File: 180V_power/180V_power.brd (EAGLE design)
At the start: 50 x 75 mm, 22 parts, among them IC1 NE555P, Q1 IRF740S, Q2 BC546

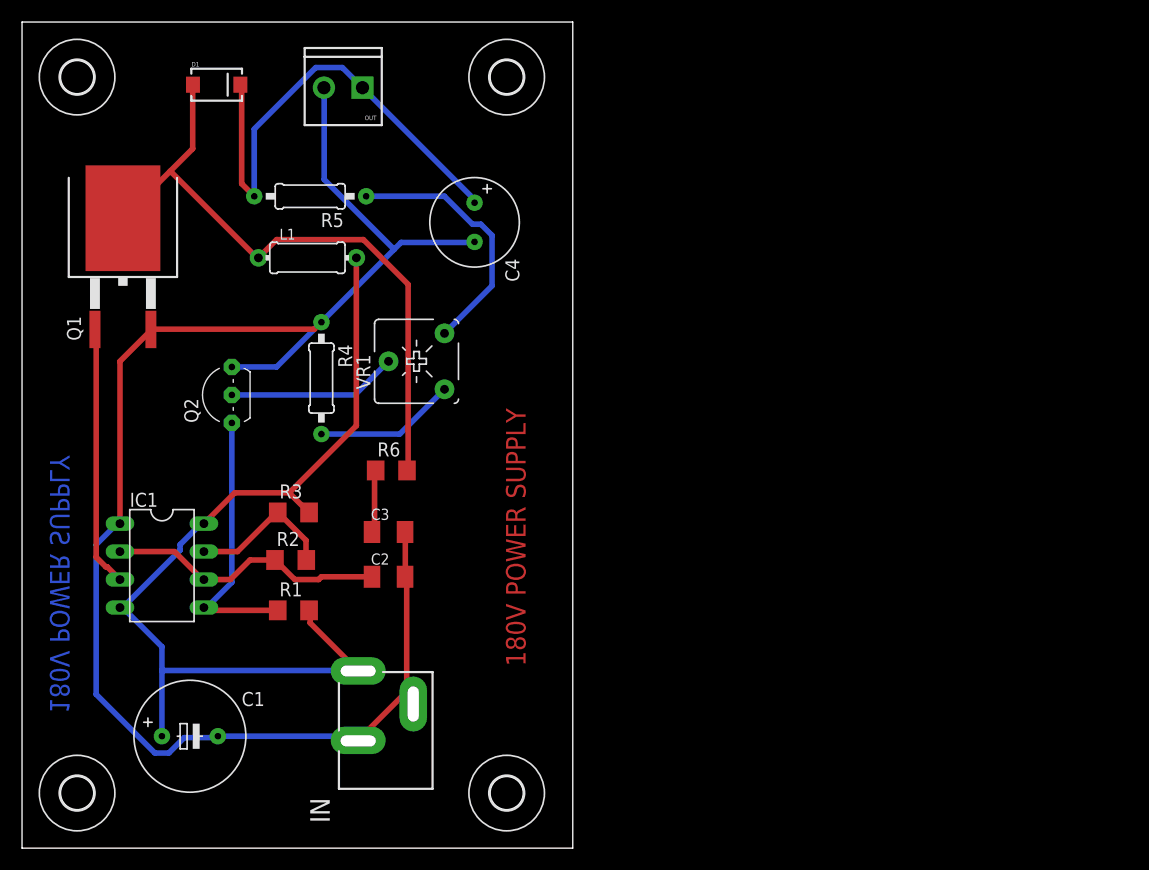
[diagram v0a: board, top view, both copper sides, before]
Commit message: new simple 180 board
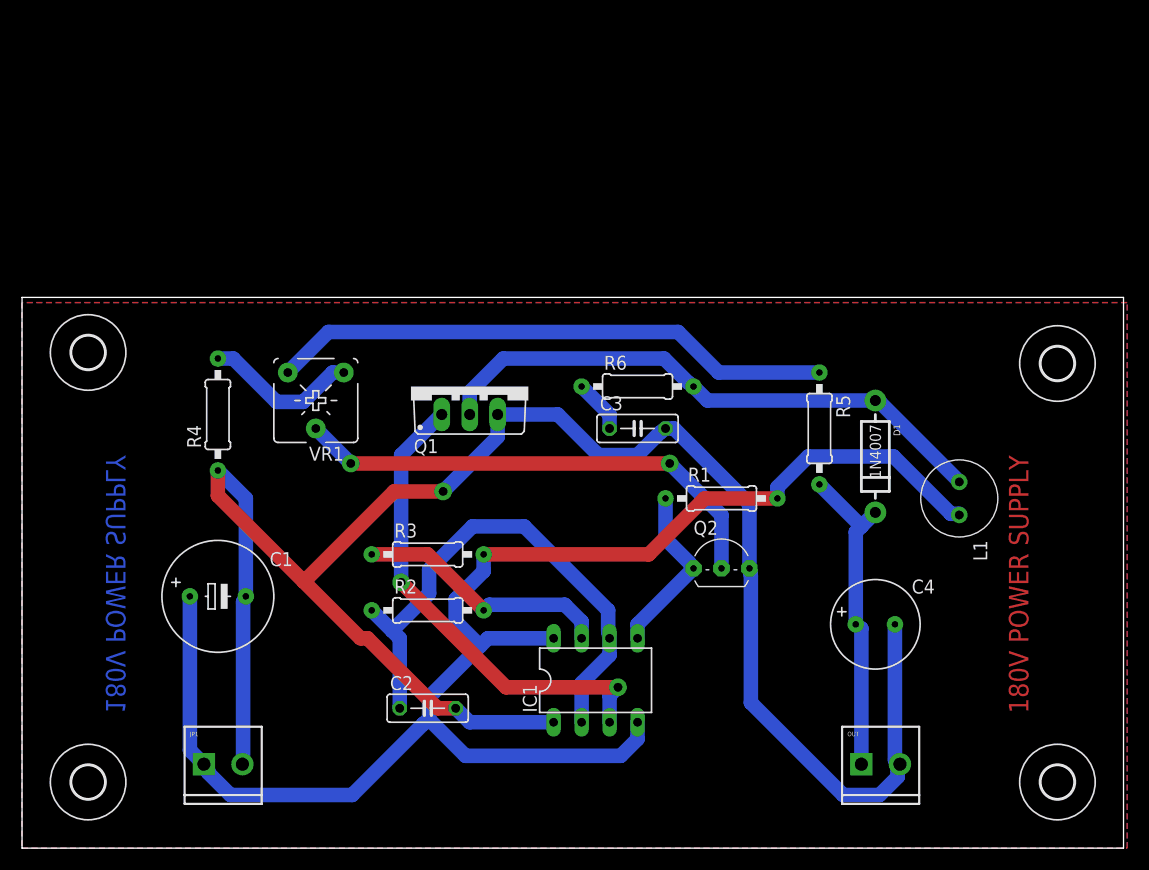
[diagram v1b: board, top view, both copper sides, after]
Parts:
- removed IN: POWER_JACKSLT, iStivi - Header-Connector:POWER_JACK_SLOT
- added JP1: (no value), iStivi - Header-Connector:SCREWTERMINAL-3.5MM-2
- C2, C3: device iStivi - RCLD:C1206K -> iStivi - RCLD:C050-025X075
- D1: device iStivi - RCLD:SMA-DIODE -> iStivi - RCLD:DIODE-1N4001
- L1: value 100uH -> (none); device iStivi - RCLD:TFI0307 -> iStivi - RCLD:RBL0712
- Q1: value IRF740S -> IRF740; device iStivi - Transistor-FET:TO263 -> iStivi - Transistor-FET:TO220BV
- R1, R2, R3, R6: device iStivi - RCLD:R1206 -> iStivi - RCLD:0207/10
- moved OUT 76.3 mm to (76.2, 7.62), turned to 0 degrees
- moved D1 68.7 mm to (77.5, 35.6), turned to 270 degrees
- moved L1 63.1 mm to (85.1, 31.8), turned to 270 degrees
- moved U$3 56.4 mm to (94.0, 44.0)
- moved C4 51.5 mm to (77.5, 20.3), turned to 0 degrees
- moved R5 50.8 mm to (72.4, 38.1), turned to 270 degrees
- moved U$2 50.0 mm to (94.0, 6.00)
- moved Q2 48.0 mm to (63.5, 26.7), turned to 0 degrees
- moved IC1 40.7 mm to (52.1, 15.2), turned to 0 degrees
- moved R1 40.2 mm to (63.5, 31.8)
- moved Q1 33.6 mm to (40.6, 41.9)
- moved U$4 25.0 mm to (6.00, 45.0)
- moved C3 24.5 mm to (55.9, 38.1)
- moved R6 23.6 mm to (55.9, 41.9)
- moved R2 13.3 mm to (36.8, 21.6)
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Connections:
- net GND: now also JP1.2, Q1.S; no longer IN.GND@1, IN.GND@2, Q1.2
- net N$1: now also Q1.G; no longer Q1.1
- net N$26: now also JP1.1, L1.P$2; no longer IN.PWR, L1.2
- net N$6: now also L1.P$1, Q1.D; no longer L1.1, Q1.3
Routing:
- net N$26: track 85.0 -> 138.4 mm
- net N$10: track 15.5 -> 44.9 mm, vias 0 -> 2
- net N$8: track 23.6 -> 51.3 mm
- net GND: track 145.2 -> 172.0 mm, vias 0 -> 1
- net N$5: track 25.5 -> 49.1 mm
- net N$1: track 23.7 -> 43.9 mm, vias 0 -> 2
- net N$7: track 44.3 -> 29.2 mm
- net N$4: track 13.6 -> 23.5 mm
- net N$3: track 24.8 -> 15.8 mm
- net N$6: track 59.0 -> 52.3 mm
- net N$9: track 12.9 -> 14.2 mm
- net N$2: track 5.85 -> 4.86 mm
- added copper zone on layer 1, net GND
- added copper zone on layer 16, net GND
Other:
- board size 50 x 75 mm -> 100 x 50 mm
- board text removed: "100uH"
- board text removed: "180V"
- board text removed: "9-12V"
- board text removed: "GND"
- board text removed: "IRF740"
- board text removed: "NE555"
